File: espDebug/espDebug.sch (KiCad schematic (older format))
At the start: 12 parts, among them P1 RAW, P2 3V3, P3 RX/TX, U1 SPX2920T-3.3, U2 ESP-201, U3 ESP8266, U4 button

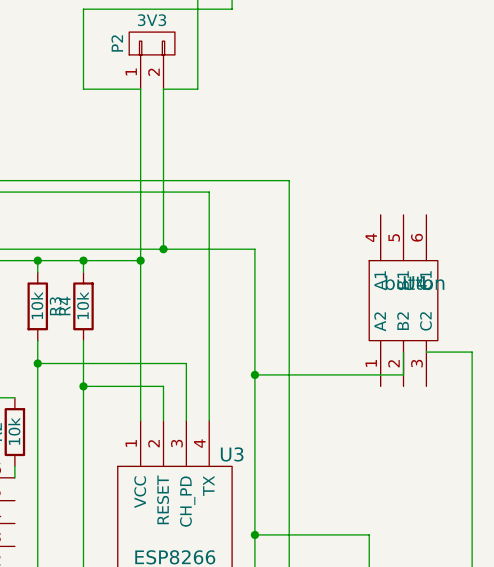
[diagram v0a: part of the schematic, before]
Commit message: CleanUp
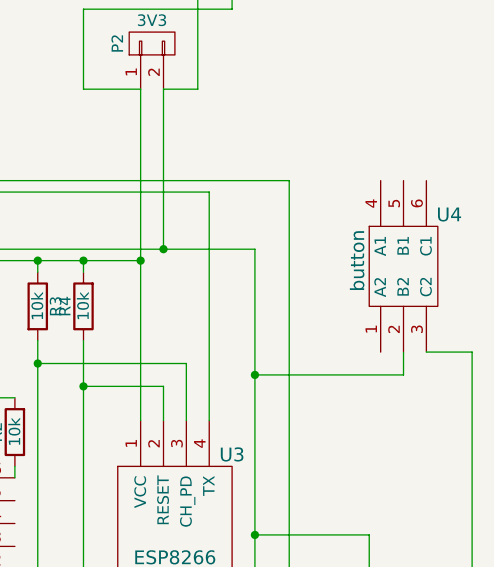
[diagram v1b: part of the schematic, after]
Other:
- moved on the sheet: U4
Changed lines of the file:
@@
 Wire Wire Line
 	3050 3850 6550 3850
-$Comp
-L button U4
-U 1 1 571AAEA1
-P 6250 1500
-F 0 "U4" H 6300 1500 60  0000 C CNN
-F 1 "button" H 6300 1500 60  0000 C CNN
-F 2 "bugs:button" H 6300 1500 60  0001 C CNN
-F 3 "" H 6300 1500 60  0000 C CNN
-	1    6250 1500
-	1    0    0    -1
-$EndComp
 Wire Wire Line
 	6550 1800 6350 1800
@@
 Wire Wire Line
 	4850 1750 4850 2850
+$Comp
+L button U4
+U 1 1 571AAEA1
+P 6250 1350
+F 0 "U4" H 6450 1500 60  0000 C CNN
+F 1 "button" V 6050 1300 60  0000 C CNN
+F 2 "bugs:button" H 6300 1350 60  0001 C CNN
+F 3 "" H 6300 1350 60  0000 C CNN
+	1    6250 1350
+	1    0    0    -1
+$EndComp
 $EndSCHEMATC
